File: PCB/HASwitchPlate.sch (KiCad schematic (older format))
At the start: 5 parts, among them J1 Screw Term., J2 XH2.54-4P, J3 Breakout, U1 IRM-03-5, U2 WeMos_mini

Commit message: PCB v0.06
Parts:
- J1: symbol Screw_Terminal_01x02 -> HASwitchPlate-library:Screw_Terminal_01x02-HASwitchPlate-library
- J2: symbol XH2.54-4P -> HASwitchPlate-library:XH2.54-4P-HASwitchPlate-library
- J3: symbol Conn_01x08 -> HASwitchPlate-library:Conn_01x08-conn-HASwitchPlate
- U1: symbol IRM-03-5 -> HASwitchPlate-library:IRM-03-5-HASwitchPlate-library
- U2: symbol WeMos_mini -> HASwitchPlate-library:WeMos_mini-HASwitchPlate
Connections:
- wire segments 49 -> 53
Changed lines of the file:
@@
-EESchema Schematic File Version 2
-LIBS:HASwitchPlate-library
-LIBS:power
-LIBS:device
-LIBS:switches
-LIBS:relays
-LIBS:motors
-LIBS:transistors
-LIBS:conn
-LIBS:linear
-LIBS:regul
-LIBS:74xx
-LIBS:cmos4000
-LIBS:adc-dac
-LIBS:memory
-LIBS:xilinx
-LIBS:microcontrollers
-LIBS:dsp
-LIBS:microchip
-LIBS:analog_switches
-LIBS:motorola
-LIBS:texas
-LIBS:intel
-LIBS:audio
-LIBS:interface
-LIBS:digital-audio
-LIBS:philips
-LIBS:display
-LIBS:cypress
-LIBS:siliconi
-LIBS:opto
-LIBS:atmel
-LIBS:contrib
-LIBS:valves
-LIBS:wemos_mini
-LIBS:ac-dc
-LIBS:Connector
+EESchema Schematic File Version 4
 LIBS:HASwitchPlate-cache
-EELAYER 25 0
+EELAYER 26 0
 EELAYER END
 $Descr A4 11693 8268
@@
 $EndDescr
 $Comp
-L WeMos_mini U2
+L HASwitchPlate-library:WeMos_mini-HASwitchPlate U2
 U 1 1 59E27669
 P 5850 3800
@@
 $EndComp
 $Comp
-L Screw_Terminal_01x02 J1
+L HASwitchPlate-library:Screw_Terminal_01x02-HASwitchPlate-library J1
 U 1 1 59E27A1F
 P 3875 3450
@@
 $EndComp
 $Comp
-L XH2.54-4P J2
+L HASwitchPlate-library:XH2.54-4P-HASwitchPlate-library J2
 U 1 1 59E297BA
 P 7150 3650
@@
 $EndComp
 $Comp
-L IRM-03-5 U1
+L HASwitchPlate-library:IRM-03-5-HASwitchPlate-library U1
 U 1 1 59E37A8B
 P 4275 3550
@@
 $EndComp
 $Comp
-L Conn_01x08 J3
+L HASwitchPlate-library:Conn_01x08-conn-HASwitchPlate J3
 U 1 1 5AB13587
 P 5750 2350
@@
 	6350 3650 6425 3650
 Wire Wire Line
-	5075 3550 5350 3550
-Wire Wire Line
-	5075 3450 5350 3450
+	5075 3550 5200 3550
+Wire Wire Line
+	5075 3450 5200 3450
 Wire Wire Line
 	5350 3650 5300 3650
@@
 	6525 3650 6950 3650
 Wire Wire Line
-	5200 3200 6525 3200
+	5200 3200 5550 3200
 Wire Wire Line
 	6525 3200 6525 3450
@@
 Text Label 4075 3450 0    60   ~ 0
 AC_L
+Wire Wire Line
+	5200 3550 5275 3550
+Wire Wire Line
+	5200 3450 5350 3450
+Wire Wire Line
+	5275 3550 5350 3550
+Wire Wire Line
+	5550 3200 6525 3200
 $EndSCHEMATC

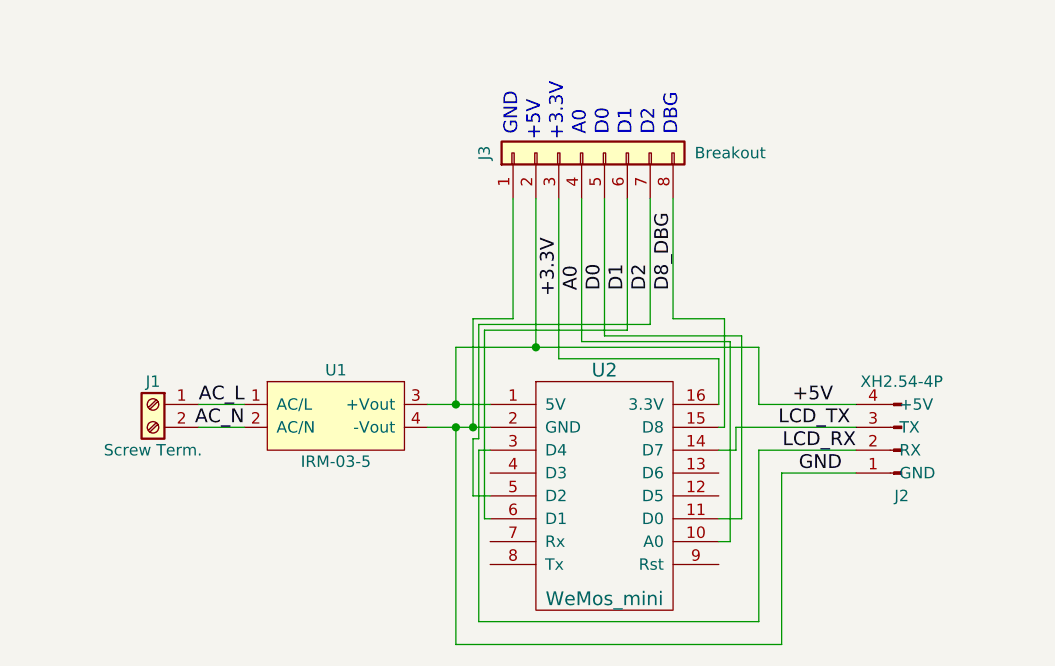
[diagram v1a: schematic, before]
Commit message: HASP v0.35
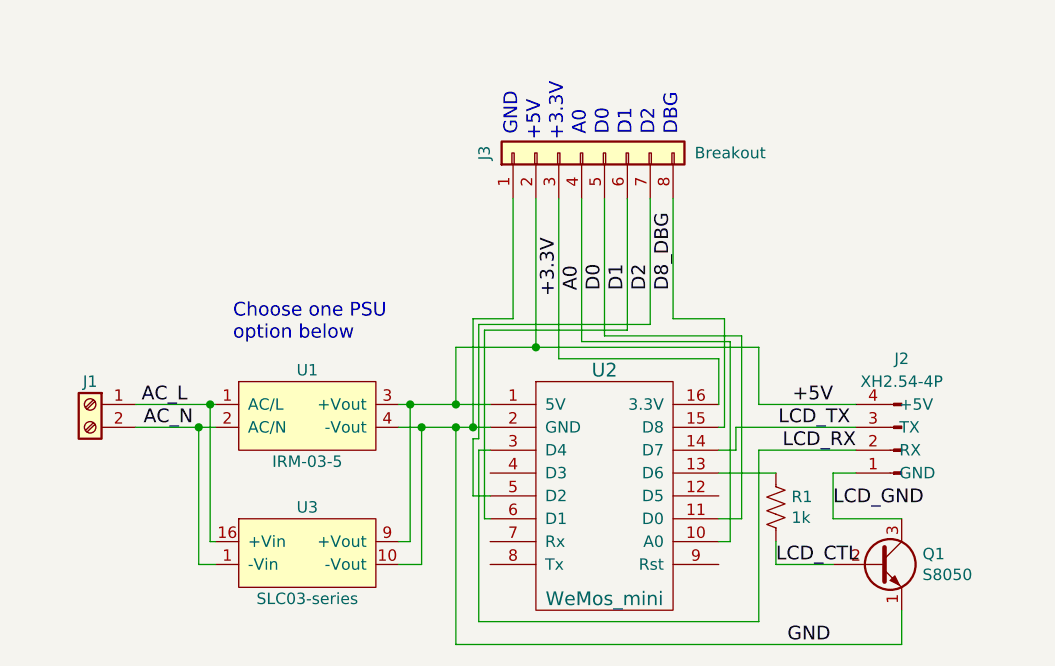
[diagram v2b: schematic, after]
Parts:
- added Q1: S8050, Package_TO_SOT_THT:TO-92L_HandSolder, symbol Transistor_BJT:S8050
- added R1: 1k, Resistor_THT:R_Axial_DIN0207_L6.3mm_D2.5mm_P7.62mm_Horizontal, symbol Device:R_US
- added U3: SLC03-series, HASwitchPlate:ACDC-Converter_MeanWell-SLC03-series, symbol HASwitchPlate-library:SLC03-series
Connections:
- net +5V: now also U3.9 (+Vout)
- net AC_L: now also U3.16 (+Vin)
- net AC_N: now also U3.1 (-Vin)
- net GND: now also Q1.1 (E), U3.10 (-Vout); no longer J2.1 (GND)
- net at U2.13 (D6): now also R1.1
- new net LCD_CTL: Q1.2 (B), R1.2
- new net LCD_GND: J2.1 (GND), Q1.3 (C)
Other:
- note added: "Choose one PSU\noption below"
- moved on the sheet: J1, U1
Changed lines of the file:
@@
 L HASwitchPlate-library:Screw_Terminal_01x02-HASwitchPlate-library J1
 U 1 1 59E27A1F
-P 3875 3450
-F 0 "J1" H 3875 3550 50  0000 C CNN
-F 1 "Screw Term." H 3875 3250 50  0000 C CNN
-F 2 "Connectors_Terminal_Blocks:TerminalBlock_bornier-2_P5.08mm" H 3875 3450 50  0001 C CNN
-F 3 "" H 3875 3450 50  0001 C CNN
-	1    3875 3450
+P 3600 3450
+F 0 "J1" H 3600 3550 50  0000 C CNN
+F 1 "Screw Term." H 3600 3250 50  0001 C CNN
+F 2 "Connectors_Terminal_Blocks:TerminalBlock_bornier-2_P5.08mm" H 3600 3450 50  0001 C CNN
+F 3 "" H 3600 3450 50  0001 C CNN
+	1    3600 3450
 	-1   0    0    -1
 $EndComp
@@
 U 1 1 59E297BA
 P 7150 3650
-F 0 "J2" H 7150 3850 50  0000 C CNN
+F 0 "J2" H 7150 3250 50  0000 C CNN
 F 1 "XH2.54-4P" H 7150 3350 50  0000 C CNN
 F 2 "HASwitchPlate:JST_XH2.54_04x2.54mm_Straight" H 7150 3650 50  0001 C CNN
@@
 L HASwitchPlate-library:IRM-03-5-HASwitchPlate-library U1
 U 1 1 59E37A8B
-P 4275 3550
-F 0 "U1" H 4675 3800 50  0000 C CNN
-F 1 "IRM-03-5" H 4675 3400 50  0000 C CNN
-F 2 "HASwitchPlate:ACDC-Converter_MeanWell-IRM-03-x" H 4675 3300 50  0001 C CNN
-F 3 "" H 4675 3200 50  0001 C CNN
-	1    4275 3550
+P 4150 3550
+F 0 "U1" H 4550 3800 50  0000 C CNN
+F 1 "IRM-03-5" H 4550 3400 50  0000 C CNN
+F 2 "HASwitchPlate:ACDC-Converter_MeanWell-IRM-03-x" H 4550 3300 50  0001 C CNN
+F 3 "https://www.meanwell.com/Upload/PDF/IRM-03/IRM-03-SPEC.PDF" H 4550 3200 50  0001 C CNN
+	1    4150 3550
 	1    0    0    -1
 $EndComp
@@
 Text Notes 6175 2275 1    60   ~ 0
 DBG
-Text Label 6700 3750 0    60   ~ 0
+Text Label 6650 4500 0    60   ~ 0
 GND
 Text Label 6950 3650 2    60   ~ 0
@@
 	6350 3650 6425 3650
 Wire Wire Line
-	5075 3550 5200 3550
-Wire Wire Line
-	5075 3450 5200 3450
+	4950 3550 5050 3550
+Wire Wire Line
+	4950 3450 5000 3450
 Wire Wire Line
 	5350 3650 5300 3650
@@
 Wire Wire Line
 	5200 3550 5200 4500
-Wire Wire Line
-	5200 4500 6625 4500
-Wire Wire Line
-	6625 4500 6625 3750
 Connection ~ 5200 3550
 Wire Wire Line
-	4075 3550 4275 3550
-Wire Wire Line
-	4075 3450 4275 3450
+	3800 3550 4075 3550
+Wire Wire Line
+	3800 3450 4125 3450
 Wire Wire Line
 	5200 3200 5200 3450
@@
 Wire Wire Line
 	6375 3075 6150 3075
-Wire Wire Line
-	6625 3750 6950 3750
 Wire Wire Line
 	5450 3075 5450 2550
@@
 Text Label 5650 2975 1    60   ~ 0
 +3.3V
-Text Label 4275 3550 2    60   ~ 0
+Text Label 4050 3550 2    60   ~ 0
 AC_N
-Text Label 4075 3450 0    60   ~ 0
+Text Label 3825 3450 0    60   ~ 0
 AC_L
 Wire Wire Line
@@
 Wire Wire Line
 	5550 3200 6525 3200
+$Comp
+L HASwitchPlate-library:SLC03-series U3
+U 1 1 5C2FF5D5
+P 4150 4150
+F 0 "U3" H 4550 4400 50  0000 C CNN
+F 1 "SLC03-series" H 4550 4000 50  0000 C CNN
+F 2 "HASwitchPlate:ACDC-Converter_MeanWell-SLC03-series" H 4550 3900 50  0001 C CNN
+F 3 "http://www.meanwellusa.com/productPdf.aspx?i=786" H 4550 3800 50  0001 C CNN
+	1    4150 4150
+	1    0    0    -1
+$EndComp
+Wire Wire Line
+	4125 3450 4125 4050
+Wire Wire Line
+	4125 4050 4150 4050
+Connection ~ 4125 3450
+Wire Wire Line
+	4125 3450 4150 3450
+Wire Wire Line
+	4075 3550 4075 4150
+Wire Wire Line
+	4075 4150 4150 4150
+Connection ~ 4075 3550
+Wire Wire Line
+	4075 3550 4150 3550
+Wire Wire Line
+	4950 4050 5000 4050
+Wire Wire Line
+	5000 4050 5000 3450
+Connection ~ 5000 3450
+Wire Wire Line
+	5000 3450 5200 3450
+Wire Wire Line
+	4950 4150 5050 4150
+Wire Wire Line
+	5050 4150 5050 3550
+Connection ~ 5050 3550
+Wire Wire Line
+	5050 3550 5200 3550
+$Comp
+L Transistor_BJT:S8050 Q1
+U 1 1 5C306D5D
+P 7050 4150
+F 0 "Q1" H 7241 4196 50  0000 L CNN
+F 1 "S8050" H 7241 4105 50  0000 L CNN
+F 2 "Package_TO_SOT_THT:TO-92L_HandSolder" H 7250 4075 50  0001 L CIN
+F 3 "http://www.unisonic.com.tw/datasheet/S8050.pdf" H 7050 4150 50  0001 L CNN
+	1    7050 4150
+	1    0    0    -1
+$EndComp
+$Comp
+L Device:R_US R1
+U 1 1 5C306DF8
+P 6600 3900
+F 0 "R1" H 6668 3946 50  0000 L CNN
+F 1 "1k" H 6668 3855 50  0000 L CNN
+F 2 "Resistor_THT:R_Axial_DIN0207_L6.3mm_D2.5mm_P7.62mm_Horizontal" V 6640 3890 50  0001 C CNN
+F 3 "~" H 6600 3900 50  0001 C CNN
+	1    6600 3900
+	1    0    0    -1
+$EndComp
+Wire Wire Line
+	6350 3750 6600 3750
+Wire Wire Line
+	6600 4050 6600 4150
+Wire Wire Line
+	6600 4150 6850 4150
+Wire Wire Line
+	7150 3950 6850 3950
+Wire Wire Line
+	6850 3950 6850 3750
+Wire Wire Line
+	6850 3750 6950 3750
+Text Label 6850 3900 0    60   ~ 0
+LCD_GND
+Text Label 6600 4150 0    60   ~ 0
+LCD_CTL
+Wire Wire Line
+	5200 4500 7150 4500
+Wire Wire Line
+	7150 4500 7150 4350
+Text Notes 4225 3175 0    60   ~ 0
+Choose one PSU\noption below
 $EndSCHEMATC
